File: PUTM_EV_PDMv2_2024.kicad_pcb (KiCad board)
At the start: 4 copper layers, 58 x 87.3 mm, 159 parts, among them IC1 BTS722204ESAXUMA1, IC2 BTS722204ESAXUMA1, IC3 BTS722204ESAXUMA1, IC4 BTS722204ESAXUMA1, J1 74650073R, J4 Conn_01x06, J5 UMPT-08-01-L-RA-WT-P-TR, J6 FTSH-107-01-L-DV-K-A, J7 USB_C_Receptacle_USB2.0_14P, J8 UMPT-08-01-L-RA-WT-P-TR, U1 STM32G0C1KCTxN, U2 LD1117S33TR_SOT223, U3 LM2675M-5.0/NOPB, U4 MCP2542FDxMF

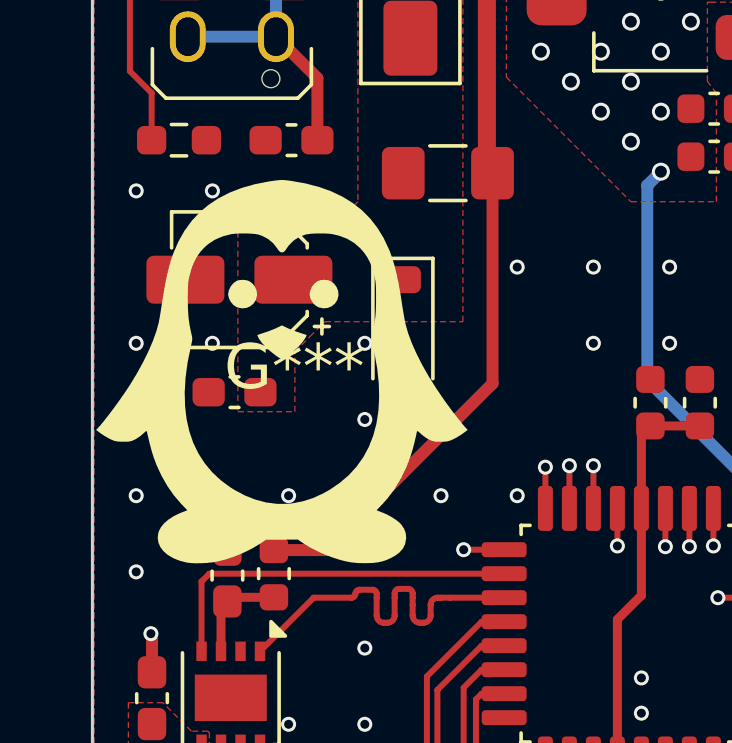
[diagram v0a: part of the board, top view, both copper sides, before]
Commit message: Production
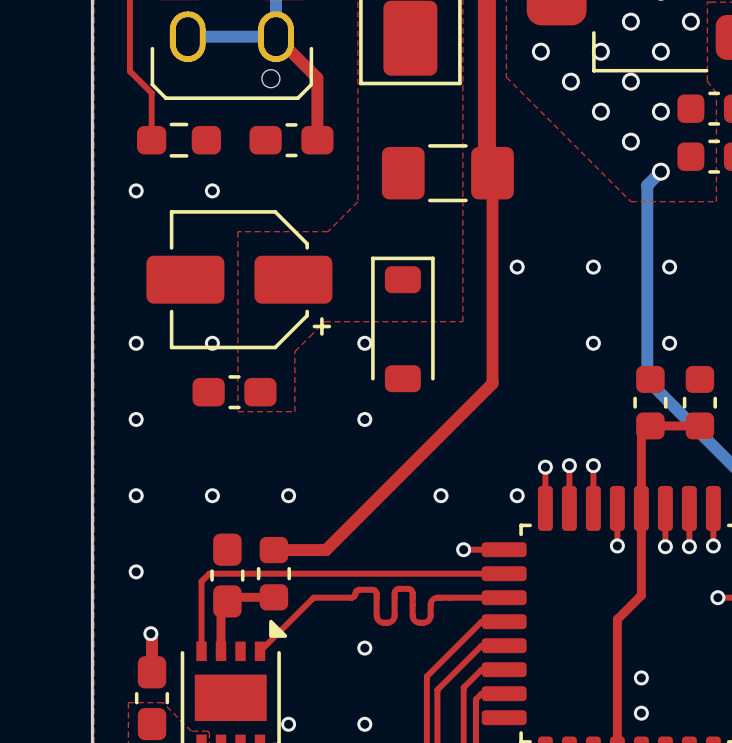
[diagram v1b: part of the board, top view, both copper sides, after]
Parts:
- removed the G*** at (127.5, 88.3)
